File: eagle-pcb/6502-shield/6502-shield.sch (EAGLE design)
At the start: 39 parts

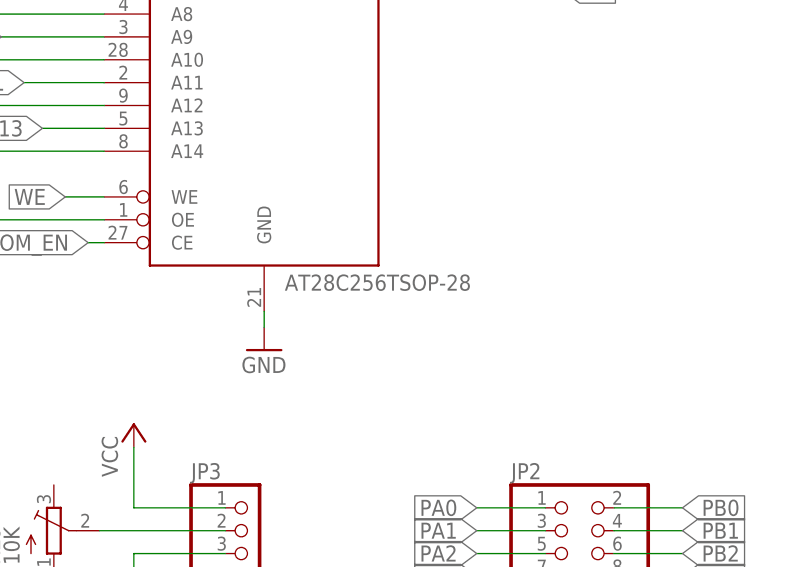
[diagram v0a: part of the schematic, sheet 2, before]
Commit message: This should be ready to send out.
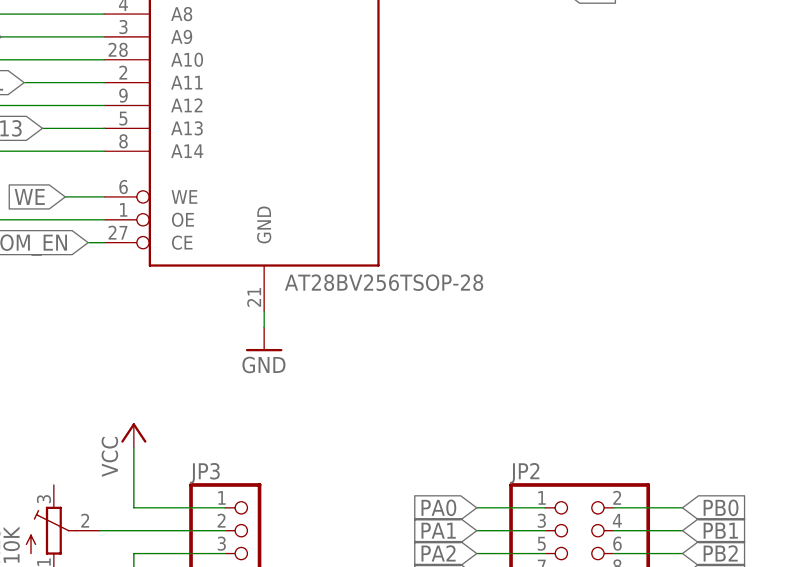
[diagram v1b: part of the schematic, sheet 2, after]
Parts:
- EEPROM: value AT28C256TSOP-28 -> AT28BV256TSOP-28; device 6502-shield:AT28C256TSOP-28 -> 6502-shield:AT28BV256TSOP-28
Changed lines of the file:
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@@
 </classes>
 <parts>
-<part name="PCB1" library="E14_Arduino_revC" library_urn="urn:adsk.eagle:library:18477430" deviceset="ARDUINO_MEGA2560" device="" package3d_urn="urn:adsk.eagle:package:18477461/4"/>
+<part name="PCB1" library="E14_Arduino_revC" library_urn="urn:adsk.eagle:library:18477430" deviceset="ARDUINO_MEGA2560" device="" package3d_urn="urn:adsk.eagle:package:18477461/5"/>
 <part name="PB_RESET" library="6502-shield" library_urn="urn:adsk.eagle:library:18477216" deviceset="MCSLPT4644B1TR-TACT-SW" device="" package3d_urn="urn:adsk.eagle:package:18592201/6"/>
 <part name="SW_RUNHALT" library="6502-shield" library_urn="urn:adsk.eagle:library:18477216" deviceset="PCM12SMTR-SPDT-RIGHT-ANG" device="" package3d_urn="urn:adsk.eagle:package:18622137/7"/>
@@
 <part name="P+17" library="supply1" library_urn="urn:adsk.eagle:library:371" deviceset="VCC" device=""/>
 <part name="GND19" library="supply1" library_urn="urn:adsk.eagle:library:371" deviceset="GND" device=""/>
-<part name="EEPROM" library="6502-shield" library_urn="urn:adsk.eagle:library:18477216" deviceset="AT28C256" device="TSOP-28" package3d_urn="urn:adsk.eagle:package:18436546/2"/>
+<part name="EEPROM" library="6502-shield" library_urn="urn:adsk.eagle:library:18477216" deviceset="AT28BV256" device="TSOP-28" package3d_urn="urn:adsk.eagle:package:18436546/2"/>
 <part name="FRAME2" library="frames" library_urn="urn:adsk.eagle:library:229" deviceset="FRAME_A_L" device="" value="6502-shield"/>
 <part name="P+19" library="supply1" library_urn="urn:adsk.eagle:library:371" deviceset="VCC" device=""/>
